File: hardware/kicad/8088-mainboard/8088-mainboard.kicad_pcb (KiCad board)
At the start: 2 copper layers, 163 x 137 mm, 64 parts, among them J1 POWER 5v, J2 Exp0, J3 Exp1, SW1 Reset, U1 8088_Max_Mode, U10 74LS273, U11 74LS00, U12 74LS138, U13 HM62256BLP, U14 74LS373, U15 74LS00, U2 8284, U3 74LS373, U5 74LS245, U6 8288, U7 74LS138, U8 28C256, U9 HM62256BLP, Y1 14.31818 MHz

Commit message: Update 8086-mainboard scheme
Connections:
- net /CPU/A0 renamed /A0
- net /CPU/A1 renamed /A1
- net /CPU/A10 renamed /A10
- net /CPU/A11 renamed /A11
- net /CPU/A12 renamed /A12
- net /CPU/A13 renamed /A13
- net /CPU/A14 renamed /A14
- net /CPU/A15 renamed /A15
- net /CPU/A16 renamed /A16
- net /CPU/A17 renamed /A17
- net /CPU/A18 renamed /A18
- net /CPU/A19 renamed /A19
- net /CPU/A2 renamed /A2
- net /CPU/A3 renamed /A3
- net /CPU/A4 renamed /A4
- net /CPU/A5 renamed /A5
- net /CPU/A6 renamed /A6
- net /CPU/A7 renamed /A7
- net /CPU/A8 renamed /A8
- net /CPU/A9 renamed /A9
- net /CPU/D0 renamed /D0
- net /CPU/D1 renamed /D1
- net /CPU/D2 renamed /D2
- net /CPU/D3 renamed /D3
- net /CPU/D4 renamed /D4
- net /CPU/D5 renamed /D5
- net /CPU/D6 renamed /D6
- net /CPU/D7 renamed /D7

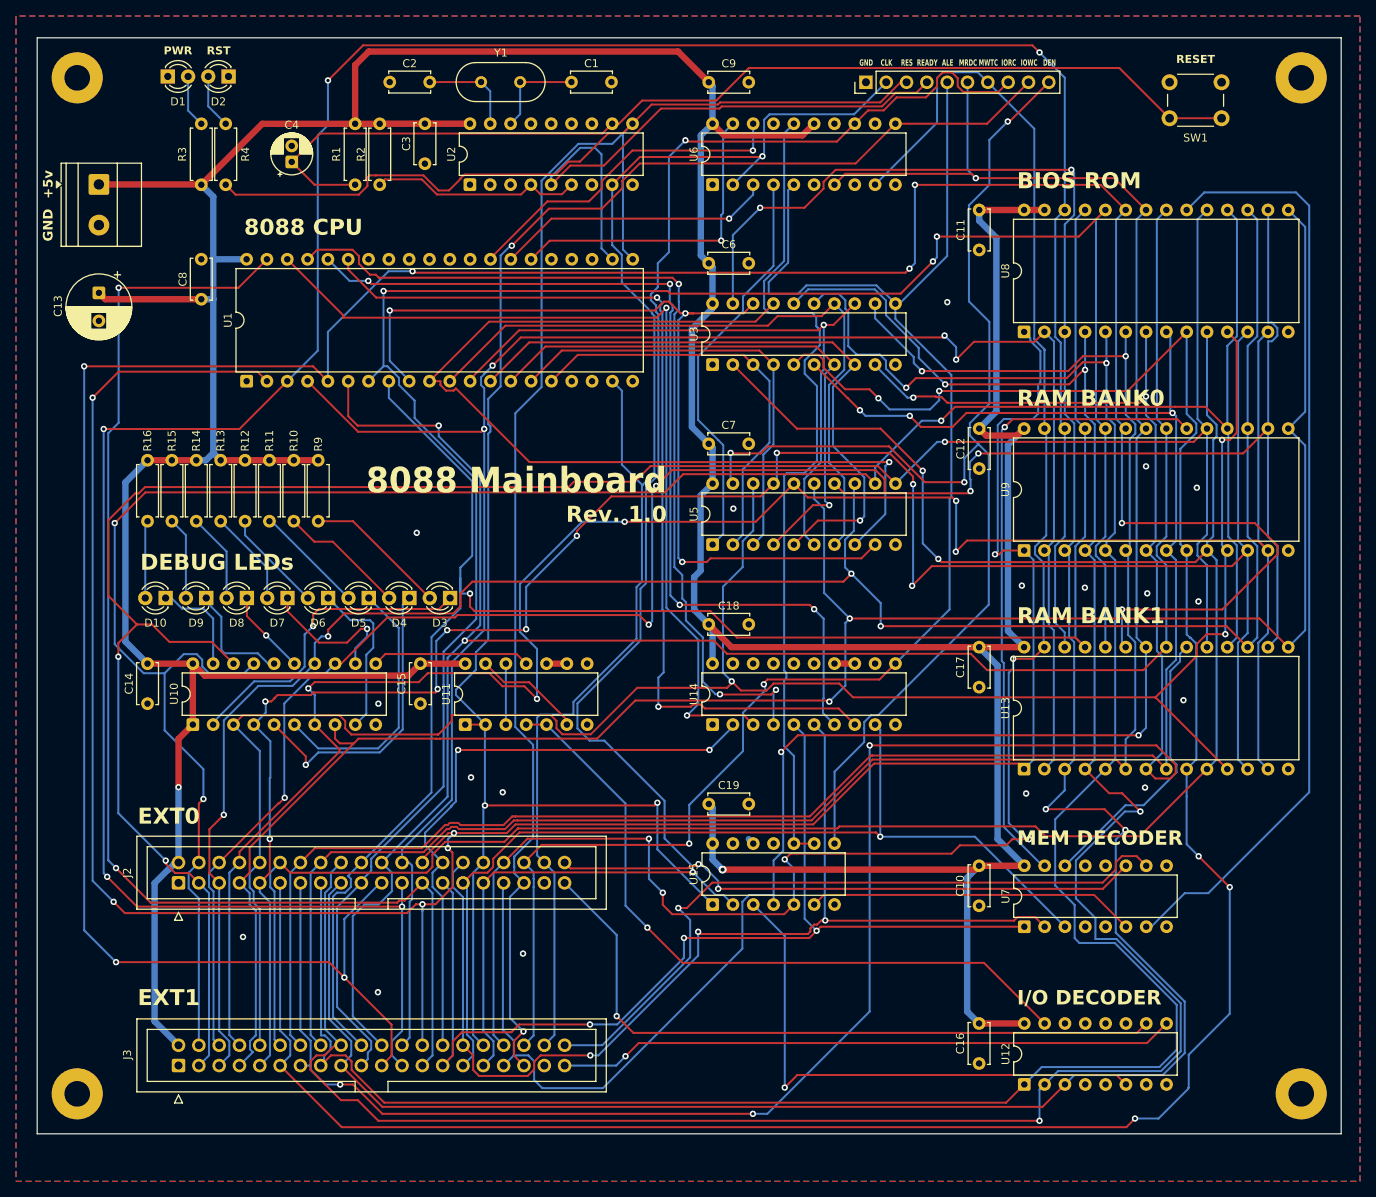
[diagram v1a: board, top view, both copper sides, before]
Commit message: Update 8086-mainboard scheme
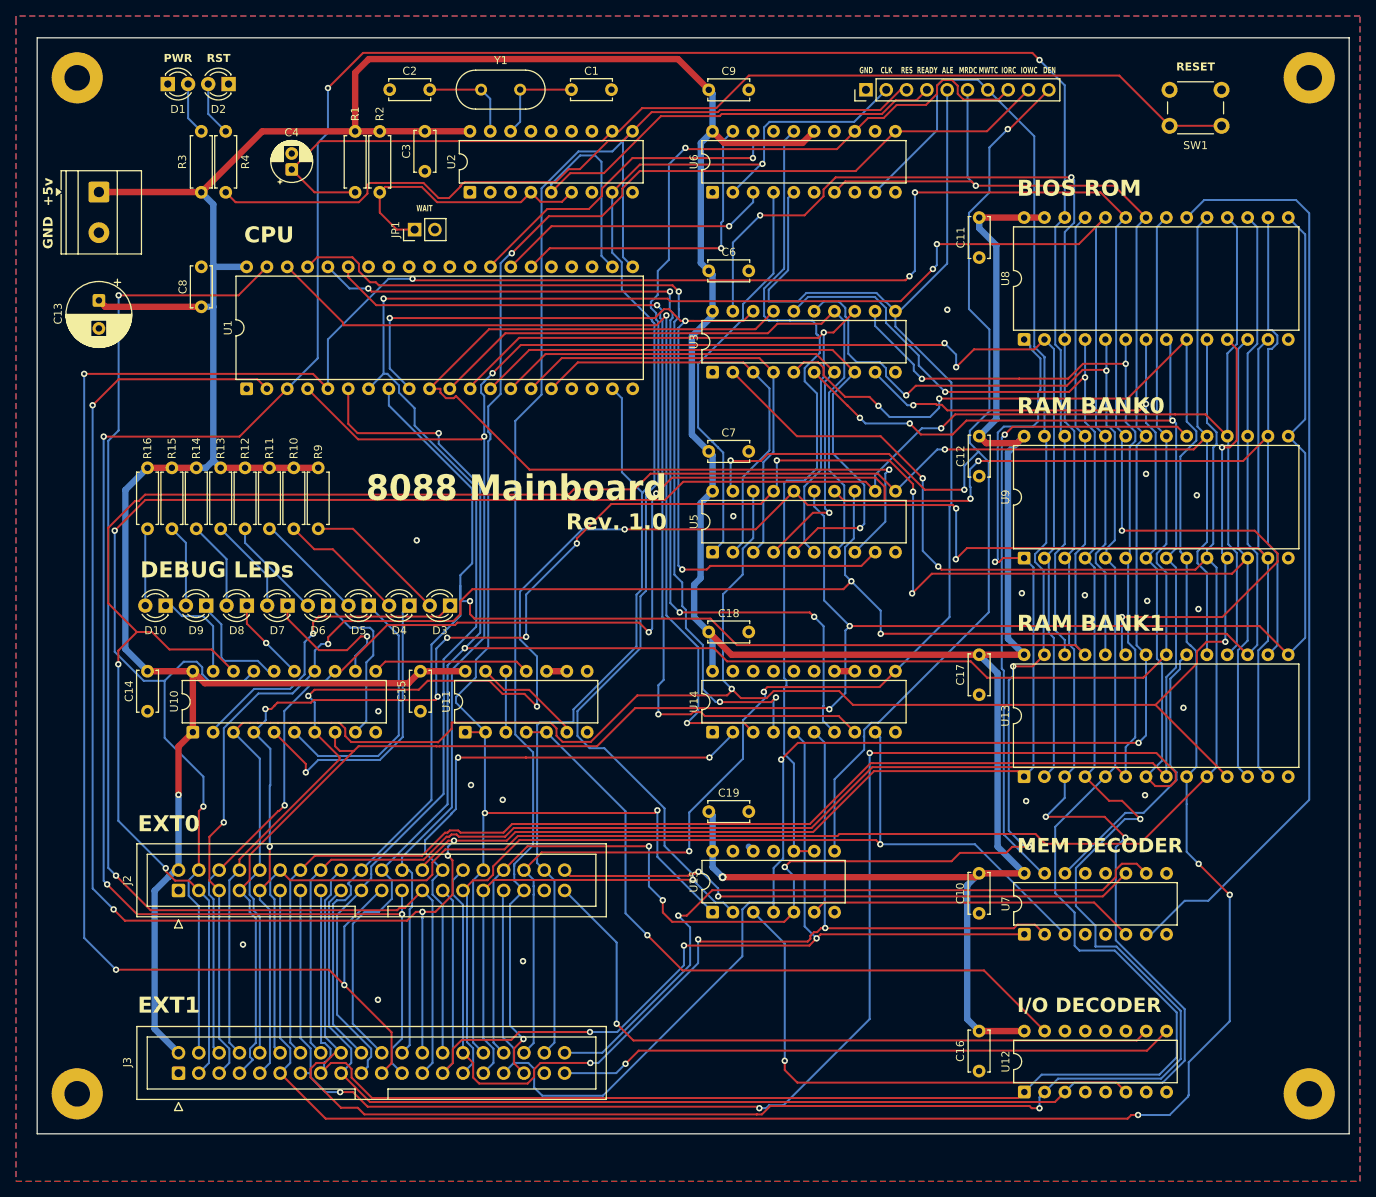
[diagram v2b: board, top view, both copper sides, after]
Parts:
- added JP1: Jumper_2_Open, Connector_PinHeader_2.54mm:PinHeader_1x02_P2.54mm_Vertical, F.Cu at (67.2, 44.0)
- moved H2 1.00 mm to (179.0, 25.0)
- moved H4 1.00 mm to (179.0, 152.0)
- moved R2 0.95 mm to (62.8, 31.7)
- moved C14 0.95 mm to (33.8, 99.2)
- moved C15 0.95 mm to (67.9, 99.2)
- moved C18 0.95 mm to (103.9, 94.3)
- moved C7 0.95 mm to (103.9, 71.7)
- moved D10 0.95 mm to (36.0, 91.0)
- moved J3 0.95 mm to (37.7, 149.4)
- moved R10 0.95 mm to (52.1, 73.7)
- moved R11 0.95 mm to (49.0, 73.7)
- moved R12 0.95 mm to (46.0, 73.7)
- moved R13 0.95 mm to (42.9, 73.7)
- moved R14 0.95 mm to (39.9, 73.7)
- moved R15 0.95 mm to (36.8, 73.7)
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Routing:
- net Net-(JP1-A): track 26.5 -> 34.3 mm
- net /IO_DEC_EN: track 68.3 -> 65.2 mm
- net /A6: track 299.0 -> 296.3 mm
- net /A1: track 301.6 -> 299.9 mm
- net /A3: track 274.6 -> 273.3 mm
- net /A7: track 316.8 -> 315.6 mm
- net /A5: track 288.0 -> 286.7 mm
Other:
- board size 163 x 137 mm -> 164 x 137 mm
- board text added: "CPU"
- board text added: "WAIT"
- board text removed: "8088 CPU"

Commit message: Update 8088-mainboard schematics
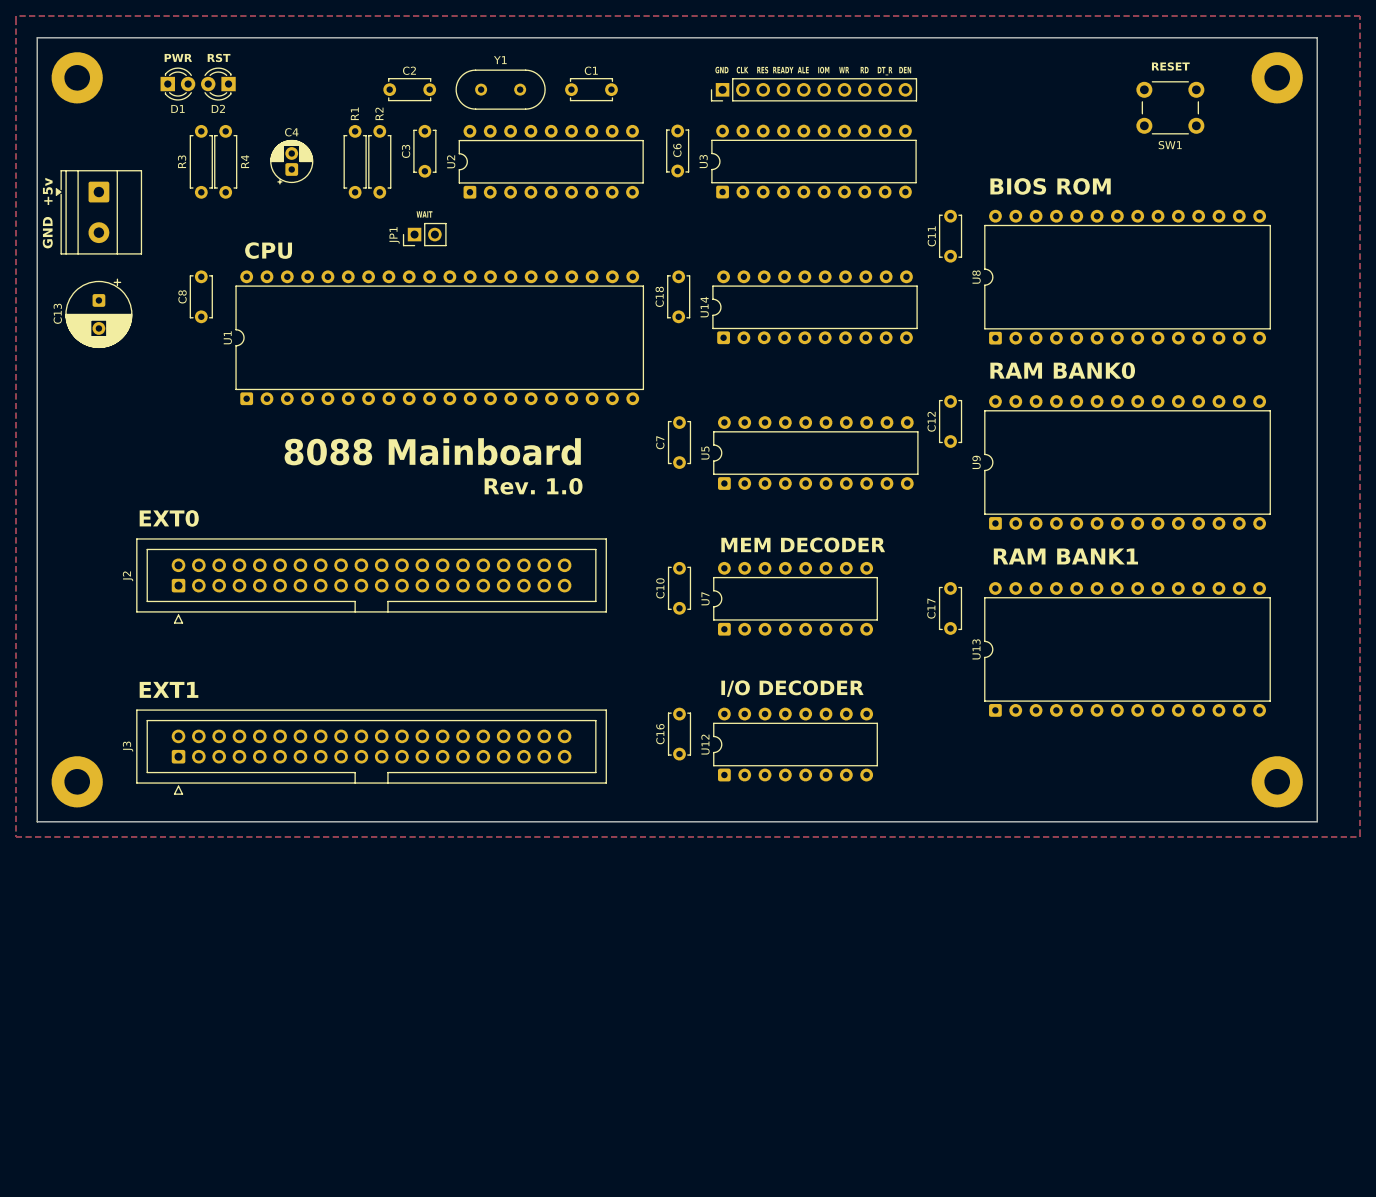
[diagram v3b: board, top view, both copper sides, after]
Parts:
- removed C14, C15, C19, C9: 100nF, Capacitor_THT:C_Disc_D5.0mm_W2.5mm_P5.00mm
- removed D10: LED7, LED_THT:LED_D3.0mm
- removed D3: LED0, LED_THT:LED_D3.0mm
- removed D4: LED1, LED_THT:LED_D3.0mm
- removed D5: LED2, LED_THT:LED_D3.0mm
- removed D6: LED3, LED_THT:LED_D3.0mm
- removed D7: LED4, LED_THT:LED_D3.0mm
- removed D8: LED5, LED_THT:LED_D3.0mm
- removed D9: LED6, LED_THT:LED_D3.0mm
- removed R10, R11, R12, R13, R14, R15, R16, R9: 680, Resistor_THT:R_Axial_DIN0207_L6.3mm_D2.5mm_P7.62mm_Horizontal
- removed U10: 74LS273, Package_DIP:DIP-20_W7.62mm
- removed U11, U15: 74LS00, Package_DIP:DIP-14_W7.62mm
- removed U6: 8288, Package_DIP:DIP-20_W7.62mm
- U1: value 8088_Max_Mode -> 8088_Min_Mode
- moved U12 54.6 mm to (105.9, 112.1)
- moved C16 54.5 mm to (100.3, 104.5)
- moved U7 53.5 mm to (105.9, 93.9)
- moved C10 53.4 mm to (100.3, 86.3)
- moved U14 49.3 mm to (105.8, 57.5)
- moved C18 44.6 mm to (100.2, 49.9), turned to -90 degrees
- moved J3 39.6 mm to (37.7, 109.9)
- moved H4 39.2 mm to (175.0, 113.0)
- moved H3 39.0 mm to (25.0, 113.0)
- moved J2 38.1 mm to (37.7, 88.5)
- moved U3 22.6 mm to (105.7, 39.3)
- moved J_DEBUG1 17.9 mm to (105.7, 26.5)
- moved C6 17.9 mm to (100.1, 31.6), turned to -90 degrees
- moved C17 9.03 mm to (134.2, 88.8)
- moved U13 9.03 mm to (139.8, 104.1)
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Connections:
- J2 pad 10: /D0 -> /A12
- J2 pad 11: /A1 -> /A11
- J2 pad 12: /A0 -> /A10
- J2 pad 13: /A3 -> /A9
- J2 pad 14: /A2 -> /A8
- J2 pad 15: /A5 -> /A7
- J2 pad 16: /A4 -> /A6
- J2 pad 17: /A7 -> /A5
- J2 pad 18: /A6 -> /A4
- J2 pad 19: /A9 -> /A3
- J2 pad 20: /A8 -> /A2
- J2 pad 21: /A11 -> /A1
- J2 pad 22: /A10 -> /A0
- J2 pad 23: /A13 -> /D7
- J2 pad 24: /A12 -> /D6
- J2 pad 25: /A15 -> /D5
- J2 pad 26: /A14 -> /D4
- J2 pad 27: /A17 -> /D3
- J2 pad 28: /A16 -> /D2
- J2 pad 29: /A19 -> /D1
- J2 pad 3: /D7 -> /A19
- J2 pad 30: /A18 -> /D0
- J2 pad 31: /IORC -> /IOM
- J2 pad 32: /IOWC -> /RD
- J2 pad 33: /MRDC -> /WR
- J2 pad 34: /MWTC -> unconnected-(J2-Pin_34-Pad34)
- J2 pad 4: /D6 -> /A18
- J2 pad 5: /D5 -> /A17
- J2 pad 6: /D4 -> /A16
- J2 pad 7: /D3 -> /A15
- J2 pad 8: /D2 -> /A14
- J2 pad 9: /D1 -> /A13
- J3 pad 10: /D0 -> /A12
- J3 pad 11: /A1 -> /A11
- J3 pad 12: /A0 -> /A10
- J3 pad 13: /A3 -> /A9
- J3 pad 14: /A2 -> /A8
- J3 pad 15: /A5 -> /A7
- J3 pad 16: /A4 -> /A6
- J3 pad 17: /A7 -> /A5
- J3 pad 18: /A6 -> /A4
- J3 pad 19: /A9 -> /A3
- J3 pad 20: /A8 -> /A2
- J3 pad 21: /A11 -> /A1
- J3 pad 22: /A10 -> /A0
- J3 pad 23: /A13 -> /D7
- J3 pad 24: /A12 -> /D6
- J3 pad 25: /A15 -> /D5
- J3 pad 26: /A14 -> /D4
- J3 pad 27: /A17 -> /D3
- J3 pad 28: /A16 -> /D2
- J3 pad 29: /A19 -> /D1
- J3 pad 3: /D7 -> /A19
- J3 pad 30: /A18 -> /D0
- J3 pad 31: /IORC -> /IOM
- J3 pad 32: /IOWC -> /RD
- J3 pad 33: /MRDC -> /WR
- J3 pad 34: /MWTC -> unconnected-(J3-Pin_34-Pad34)
- J3 pad 4: /D6 -> /A18
- J3 pad 5: /D5 -> /A17
- J3 pad 6: /D4 -> /A16
- J3 pad 7: /D3 -> /A15
- J3 pad 8: /D2 -> /A14
- J3 pad 9: /D1 -> /A13
- J_DEBUG1 pad 6: /MRDC -> /IOM
- J_DEBUG1 pad 7: /MWTC -> /WR
- J_DEBUG1 pad 8: /IORC -> /RD
- J_DEBUG1 pad 9: /IOWC -> /CPU/DT_R
- U1 pad 25: unconnected-(U1-QS0-Pad25) -> /ALE
- U1 pad 26: /CPU/S0 -> /CPU/DEN
- U1 pad 27: /CPU/S1 -> /CPU/DT_R
- U1 pad 28: /CPU/S2 -> /IOM
- U1 pad 29: unconnected-(U1-~{LOCK}-Pad29) -> /WR
- U1 pad 31: unconnected-(U1-~{RQ}/~{GT0}-Pad31) -> GND
- U1 pad 32: unconnected-(U1-~{RD}-Pad32) -> /RD
- U1 pad 33: GND -> VCC
- U12 pad 15: /IO_DECODER/LED_PANEL_CS -> unconnected-(U12-O0-Pad15)
- U12 pad 6: /IO_DEC_EN -> /IOM
- U13 pad 22: /MRDC -> /RD
- U13 pad 27: /MWTC -> /WR
- U7 pad 4: GND -> /IOM
- U7 pad 6: /MEM_DEC_EN -> VCC
- U8 pad 22: /MRDC -> /RD
- U9 pad 22: /MRDC -> /RD
- U9 pad 27: /MWTC -> /WR
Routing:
- net VCC: track 606.6 -> 0.00 mm, vias 2 -> 0
- net /A11: track 374.5 -> 0.00 mm, vias 8 -> 0
- net /A13: track 352.3 -> 0.00 mm, vias 5 -> 0
- net /A7: track 315.6 -> 0.00 mm, vias 4 -> 0
- net /A14: track 303.1 -> 0.00 mm, vias 6 -> 0
- net /A1: track 299.9 -> 0.00 mm, vias 5 -> 0
- net /A6: track 296.3 -> 0.00 mm, vias 4 -> 0
- net /D6: track 292.7 -> 0.00 mm, vias 3 -> 0
- net /D7: track 291.5 -> 0.00 mm, vias 3 -> 0
- net /A5: track 286.7 -> 0.00 mm, vias 2 -> 0
- net /A0: track 279.6 -> 0.00 mm, vias 2 -> 0
- net /A3: track 273.3 -> 0.00 mm, vias 5 -> 0
- net /D1: track 267.1 -> 0.00 mm, vias 9 -> 0
- net /A9: track 266.9 -> 0.00 mm, vias 3 -> 0
- net /D4: track 264.6 -> 0.00 mm, vias 5 -> 0
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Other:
- board size 164 x 137 mm -> 160 x 98 mm
- board text added: "DT_R"
- board text added: "IOM"
- board text added: "RD"
- board text added: "WR"
- board text removed: "DEBUG LEDs"
- board text removed: "IORC"
- board text removed: "IOWC"
- board text removed: "MRDC"
- board text removed: "MWTC"
